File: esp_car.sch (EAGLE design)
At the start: 49 parts, among them IC1 TB6612FNG, IC2 LT1963ES8-3.3, SW2 SK-12D01, U2 ESP-WROOM-32_NOFLASH

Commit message: pdf add
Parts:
- added C14: 0.1uF, rcl:C-EUC1608
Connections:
- net +5V: now also C14.1
- net GND: now also C14.2
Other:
- moved on the sheet: C10, C9, IC1, ML, MR, NDS9936A, NDS9936B, R2, SERIAL, UNIV

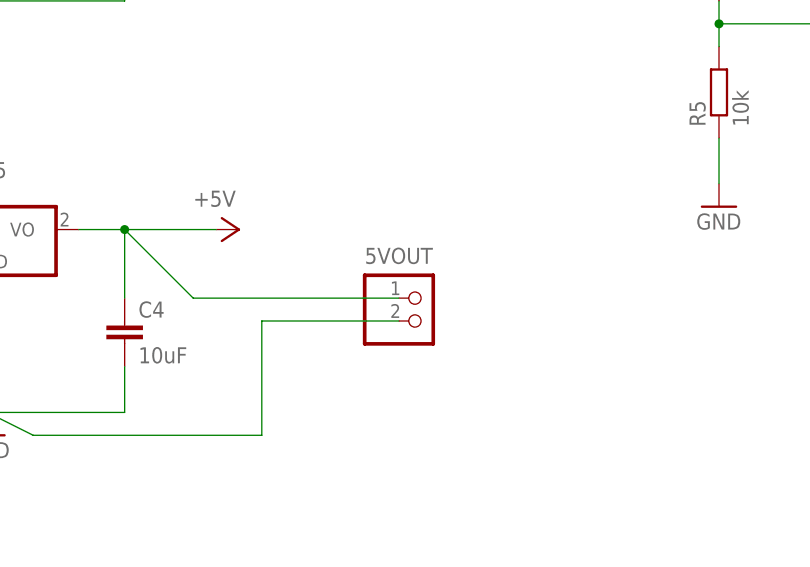
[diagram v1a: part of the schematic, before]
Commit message: from office
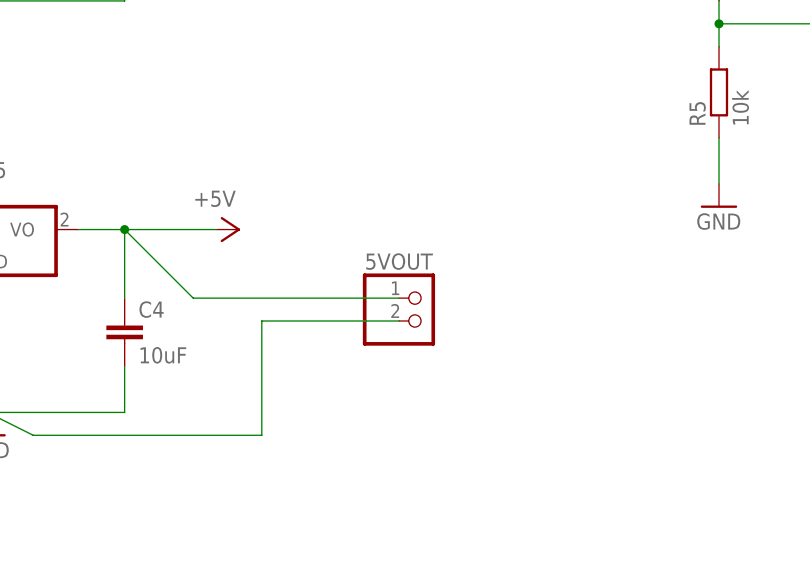
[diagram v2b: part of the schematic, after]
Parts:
- 5VOUT: device jst-xh:B2B-XH-A -> pinhead:PINHD-1X2
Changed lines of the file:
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@@
 </variantdefs>
 <classes>
-<class number="0" name="default" width="0" drill="0">
+<class number="0" name="default" width="0.4064" drill="0">
+</class>
+<class number="1" name="L" width="1.016" drill="0">
 </class>
 </classes>
@@
 <part name="R6" library="rcl" library_urn="urn:adsk.eagle:library:334" deviceset="R-EU_" device="R0603" package3d_urn="urn:adsk.eagle:package:23555/2" value="20k"/>
 <part name="UNIV" library="adafruit" deviceset="PINHD-1X9" device=""/>
-<part name="5VOUT" library="jst-xh" deviceset="B2B-XH-A" device=""/>
 <part name="BUZ+" library="wirepad" library_urn="urn:adsk.eagle:library:412" deviceset="SMD2" device="" package3d_urn="urn:adsk.eagle:package:30839/1"/>
 <part name="BUZ-" library="wirepad" library_urn="urn:adsk.eagle:library:412" deviceset="SMD2" device="" package3d_urn="urn:adsk.eagle:package:30839/1"/>
 <part name="C14" library="rcl" library_urn="urn:adsk.eagle:library:334" deviceset="C-EU" device="C1608" package3d_urn="urn:adsk.eagle:package:23621/2" value="0.1uF"/>
+<part name="5VOUT" library="pinhead" library_urn="urn:adsk.eagle:library:325" deviceset="PINHD-1X2" device="" package3d_urn="urn:adsk.eagle:package:22435/2"/>
 </parts>
 <sheets>
@@
 <instance part="R6" gate="G$1" x="60.96" y="88.9" rot="R90"/>
 <instance part="UNIV" gate="G$1" x="50.8" y="-10.16"/>
-<instance part="5VOUT" gate="G$1" x="25.4" y="50.8"/>
 <instance part="BUZ+" gate="1" x="142.24" y="58.42"/>
 <instance part="BUZ-" gate="1" x="142.24" y="53.34"/>
 <instance part="C14" gate="G$1" x="231.14" y="17.78"/>
+<instance part="5VOUT" gate="G$1" x="27.94" y="48.26"/>
 </instances>
 <busses>
 </busses>
 <nets>
-<net name="VDD" class="0">
+<net name="VDD" class="1">
 <segment>
 <pinref part="C8" gate="G$1" pin="+"/>
@@
 </segment>
 </net>
-<net name="GND" class="0">
+<net name="GND" class="1">
 <segment>
 <pinref part="GND1" gate="1" pin="GND"/>
@@
 </segment>
 </net>
-<net name="+3V3" class="0">
+<net name="+3V3" class="1">
 <segment>
 <pinref part="C1" gate="G$1" pin="1"/>
@@
 </segment>
 </net>
-<net name="+5V" class="0">
+<net name="+5V" class="1">
 <segment>
 <pinref part="NJM7805" gate="A1" pin="VO"/>
@@
 </segment>
 </net>
-<net name="VCC" class="0">
+<net name="VCC" class="1">
 <segment>
 <wire x1="-50.8" y1="111.76" x2="-50.8" y2="104.14" width="0.1524" layer="91"/>
